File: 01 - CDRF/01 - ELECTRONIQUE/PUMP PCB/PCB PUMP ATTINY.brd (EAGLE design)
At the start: 25 x 25 mm, 18 parts, among them IC1 ATTINY402-SSN, J3 PWRPAD2-5MM, J4 PWRPAD2-5MM

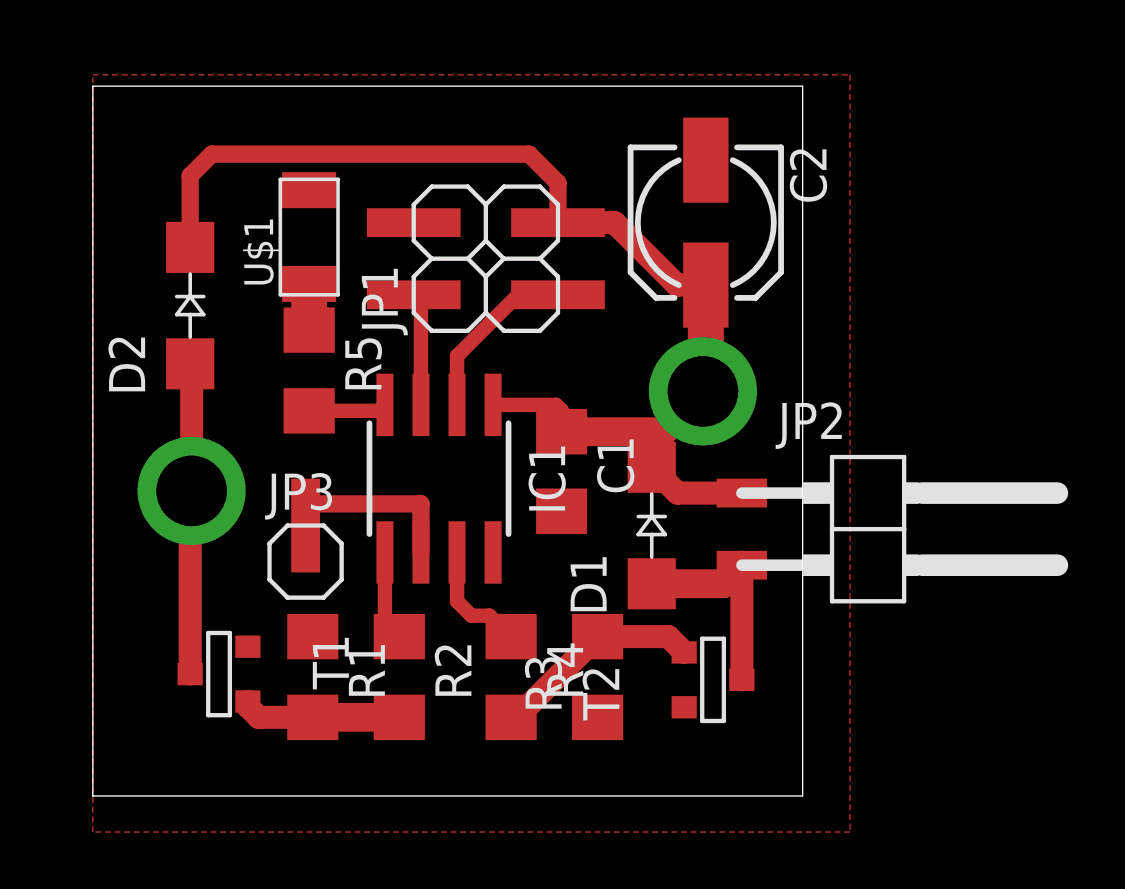
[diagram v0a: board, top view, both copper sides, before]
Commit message: Fisrt version laser
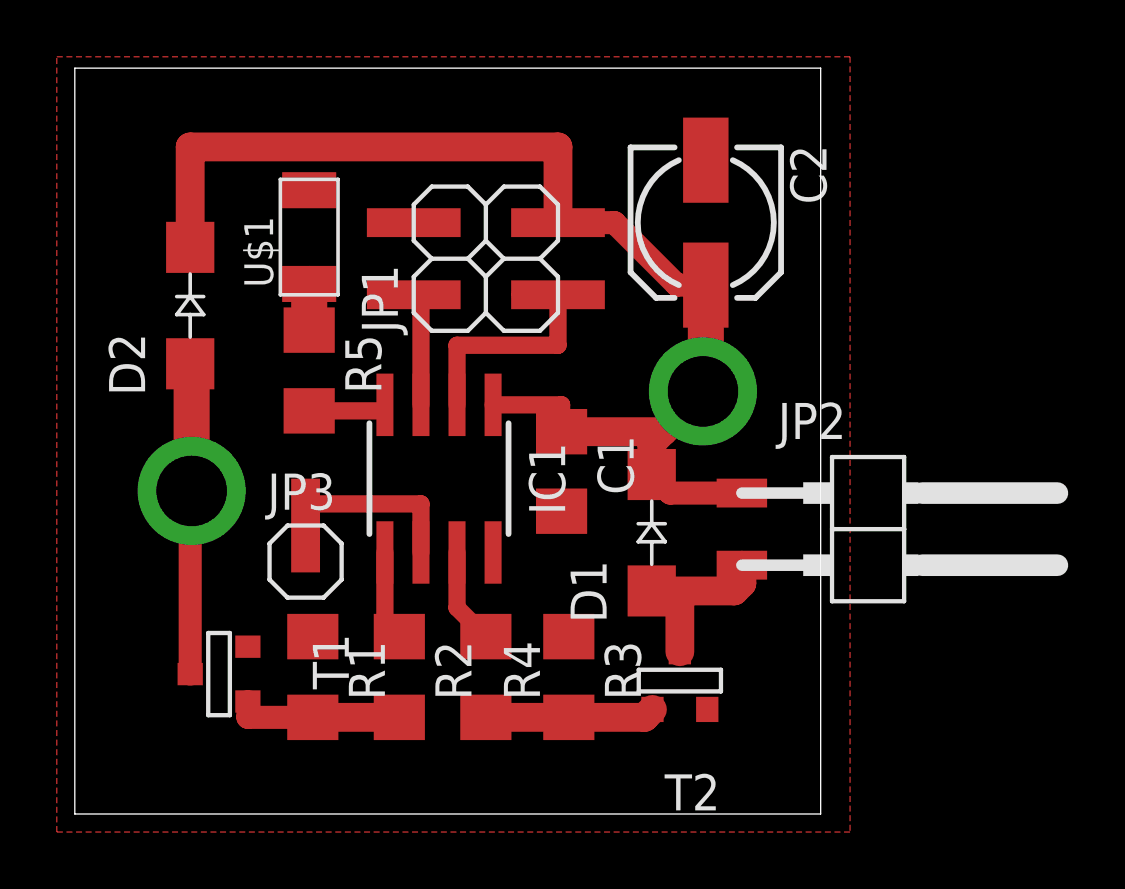
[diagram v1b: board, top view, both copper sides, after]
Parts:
- moved T2 1.14 mm to (20.7, 4.06), turned to 180 degrees
- moved R3 1.02 mm to (16.8, 4.19), turned to 270 degrees
- moved R4 0.89 mm to (13.8, 4.19)
- moved D1 0.25 mm to (19.7, 9.27)
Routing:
- net TX: track 6.17 -> 8.83 mm
- net +5V: track 43.4 -> 45.2 mm
- net N$4: track 7.51 -> 5.98 mm
- net N$1: track 7.48 -> 6.21 mm
- net EV: track 4.14 -> 3.38 mm
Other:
- board size 25 x 25 mm -> 26.3 x 26.3 mm
